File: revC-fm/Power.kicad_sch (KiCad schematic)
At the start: 29 parts, among them Q73 MUN5311DW1, U10 INA230AIRGTR, U11 BQ25883RGER, U12 INA230AIRGTR

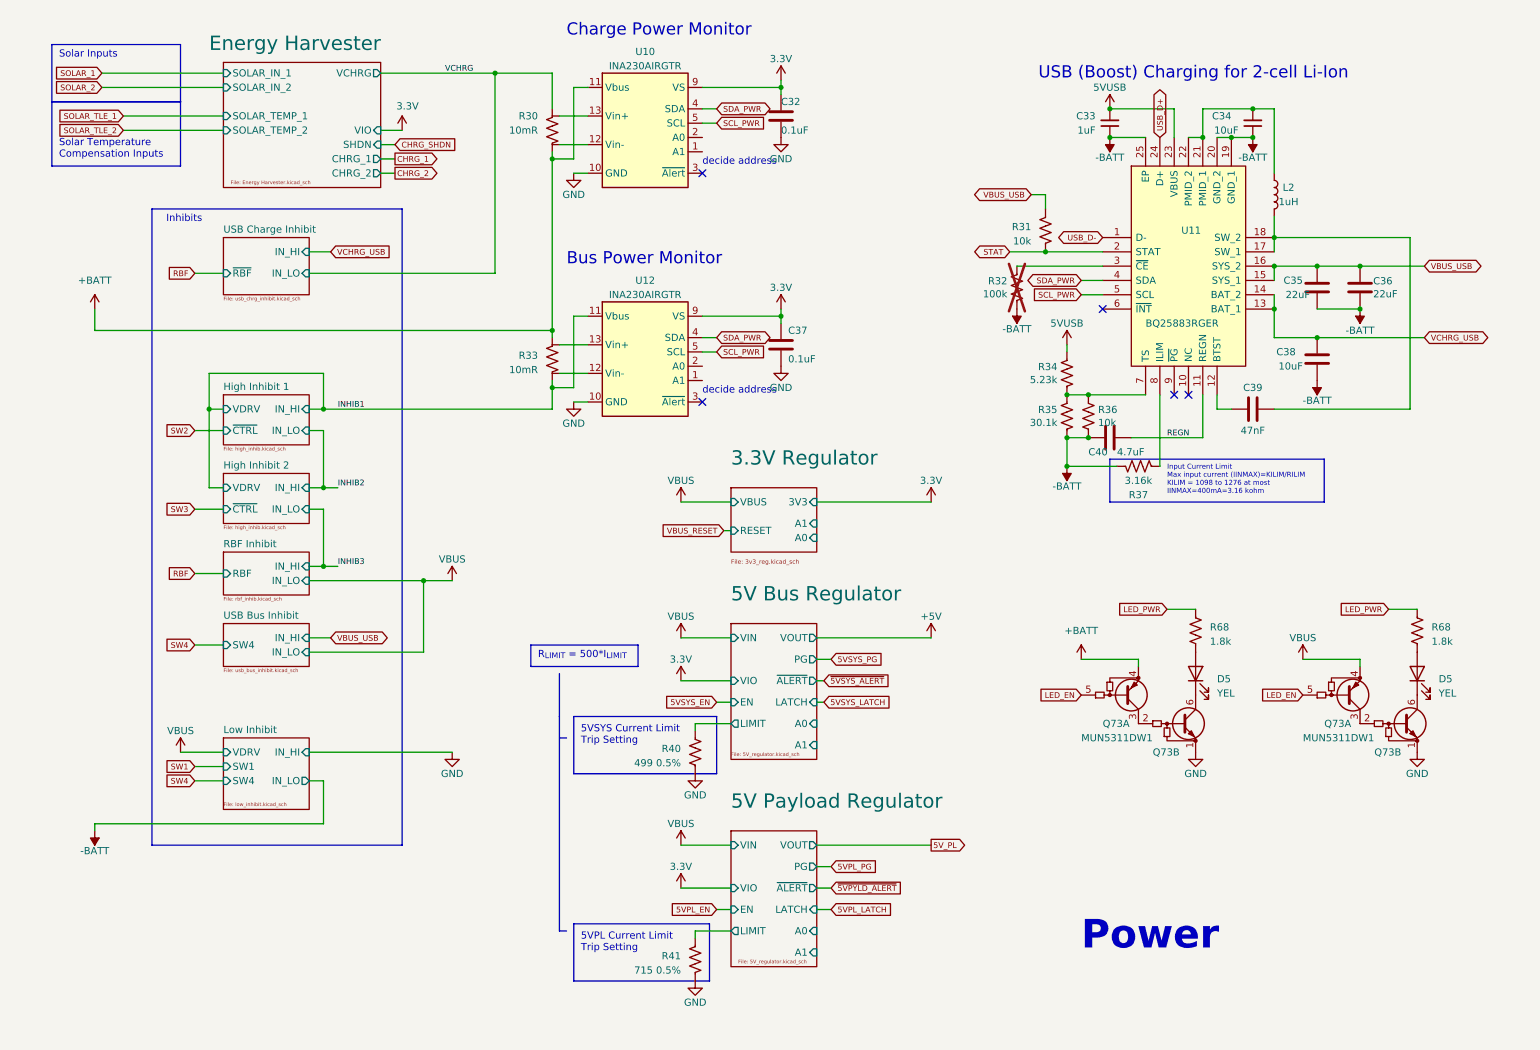
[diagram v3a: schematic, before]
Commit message: almost done!!!!!
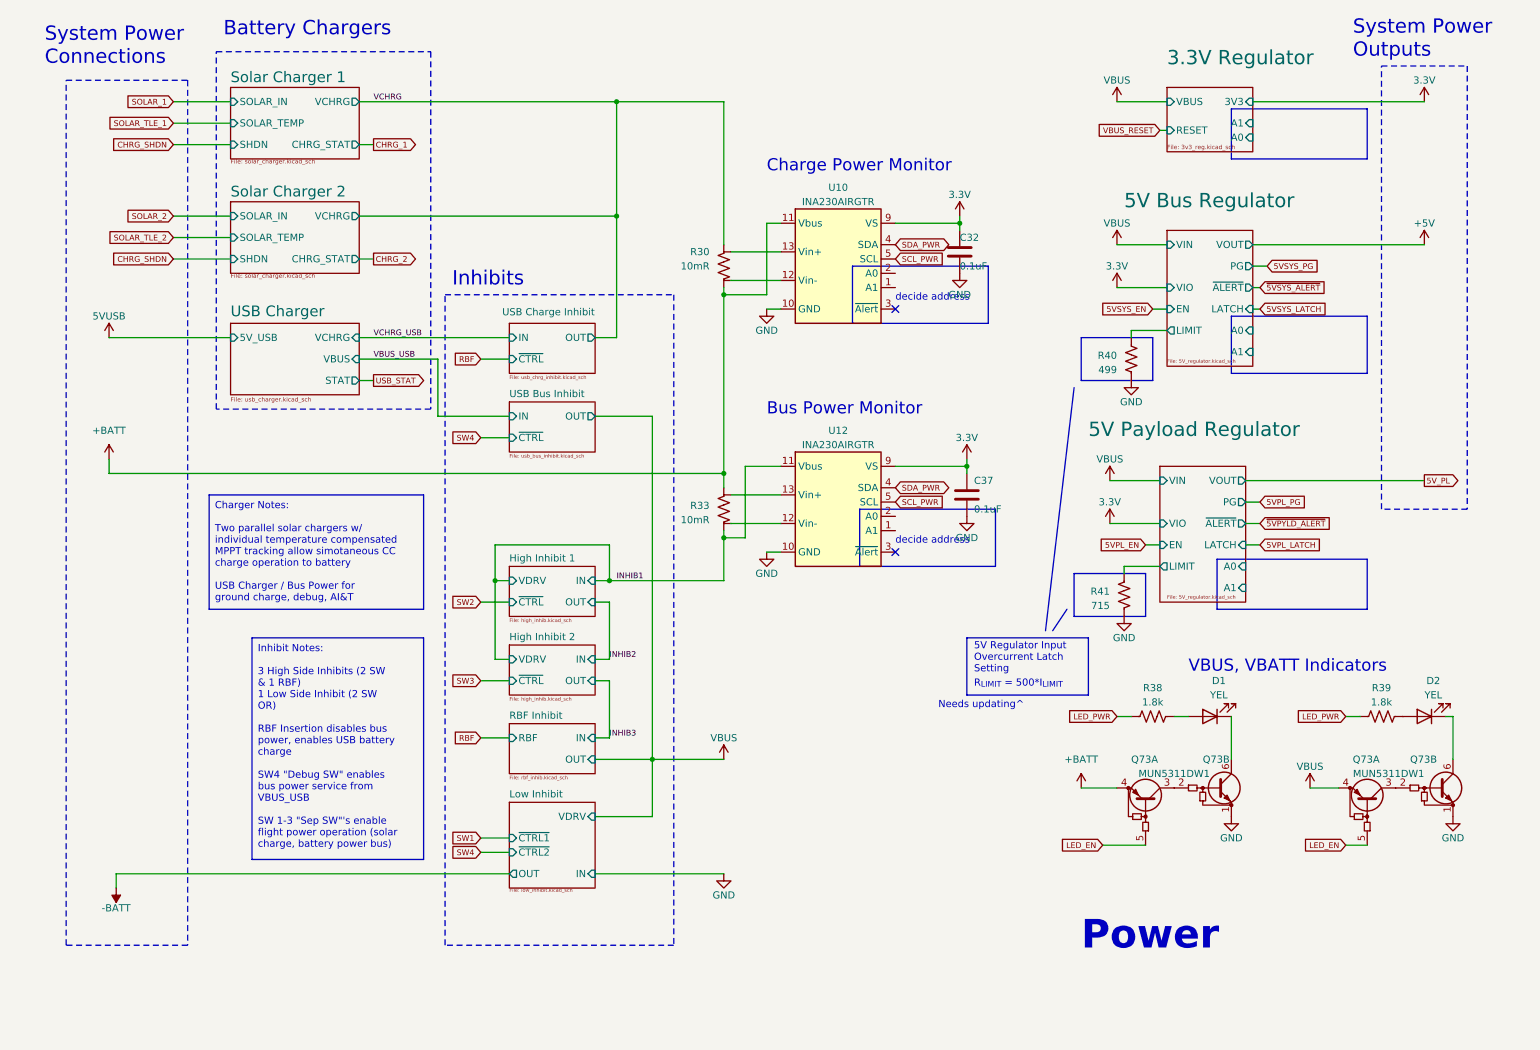
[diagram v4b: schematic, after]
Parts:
- removed C33: 1uF, Capacitor_SMD:C_0603_1608Metric, symbol Device:C_Small
- removed C34: 10uF, Capacitor_SMD:C_0805_2012Metric, symbol Device:C_Small
- removed C35, C36: 22uF, Capacitor_SMD:C_0805_2012Metric, symbol Device:C
- removed C38: 10uF, Capacitor_SMD:C_0805_2012Metric, symbol Device:C
- removed C39: 47nF, Capacitor_SMD:C_0402_1005Metric, symbol Device:C
- removed C40: 4.7uF, Capacitor_SMD:C_0603_1608Metric, symbol Device:C
- removed L2: 1uH, SierraLobo:74404032010, symbol Device:L
- removed R31, R36: 10k, Resistor_SMD:R_0402_1005Metric, symbol Device:R_US
- removed R32: 100k, Resistor_SMD:R_0402_1005Metric, symbol Device:R_US
- removed R34: 5.23k, Resistor_SMD:R_0603_1608Metric, symbol Device:R_US
- removed R35: 30.1k, Resistor_SMD:R_0603_1608Metric, symbol Device:R_US
- removed R37: 3.16k, Resistor_SMD:R_0603_1608Metric, symbol Device:R_US
- removed U11: BQ25883RGER, SierraLobo:QFN50P400X400X100-25N-D, symbol SierraLobo:BQ25883RGER
- R40: value 499 0.5% -> 499
- R41: value 715 0.5% -> 715
- renumbered D5 to D1, D5 to D2, R68 to R38, R68 to R39
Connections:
- no-connect marks 5 -> 2
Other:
- removed sheet Energy Harvester
- added sheet Solar Charger 1 (solar_charger.kicad_sch)
- added sheet Solar Charger 2 (solar_charger.kicad_sch)
- added sheet USB Charger (usb_charger.kicad_sch)
- sheet High Inhibit 1 ports: added IN, OUT; removed IN_HI, IN_LO
- sheet High Inhibit 2 ports: added IN, OUT; removed IN_HI, IN_LO
- sheet Low Inhibit ports: added IN, OUT, ~{CTRL1}, ~{CTRL2}; removed IN_HI, IN_LO, SW1, SW4
- sheet RBF Inhibit ports: added IN, OUT; removed IN_HI, IN_LO
- sheet USB Bus Inhibit ports: added IN, OUT, ~{CTRL}; removed IN_HI, IN_LO, SW4
- sheet USB Charge Inhibit ports: added IN, OUT, ~{CTRL}; removed IN_HI, IN_LO, ~{RBF}
- note added: "5V Regulator Input Overcurrent Latch Setting"
- note added: "Battery Chargers"
- note added: "Needs updating^"
- note added: "System Power Connections"
- note added: "System Power Outputs"
- note added: "VBUS, VBATT Indicators"
- note removed: "5VPL Current Limit Trip Setting"
- note removed: "5VSYS Current Limit Trip Setting"
- note removed: "Input Current Limit Max input current (IINMAX)=KILIM/RILIM KILIM = 1098 to 1276 at most IINMAX=400mA=3.16 kohm"
- note removed: "Solar Inputs"
- note removed: "Solar Temperature Compensation Inputs"
- note removed: "USB (Boost) Charging for 2-cell Li-Ion"
- moved on the sheet: C32, C37, D1, D2, Q73A, Q73B, R30, R33, R38, R39, R40, R41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
